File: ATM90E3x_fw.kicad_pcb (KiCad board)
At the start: 2 copper layers, 50.8 x 50.8 mm, 67 parts, among them IC1 ATM90E36_ATM90E36, J1 RJ45, J2 CONN_01X04, J3 GS3, J4 GS3, J5 GS3, J6 CONN_01X06, J7 CONN_01X06, J8 CONN_01X04, J9 GROVE-SMD-90D, U1 ROF-78E, Y1 Crystal_GND24

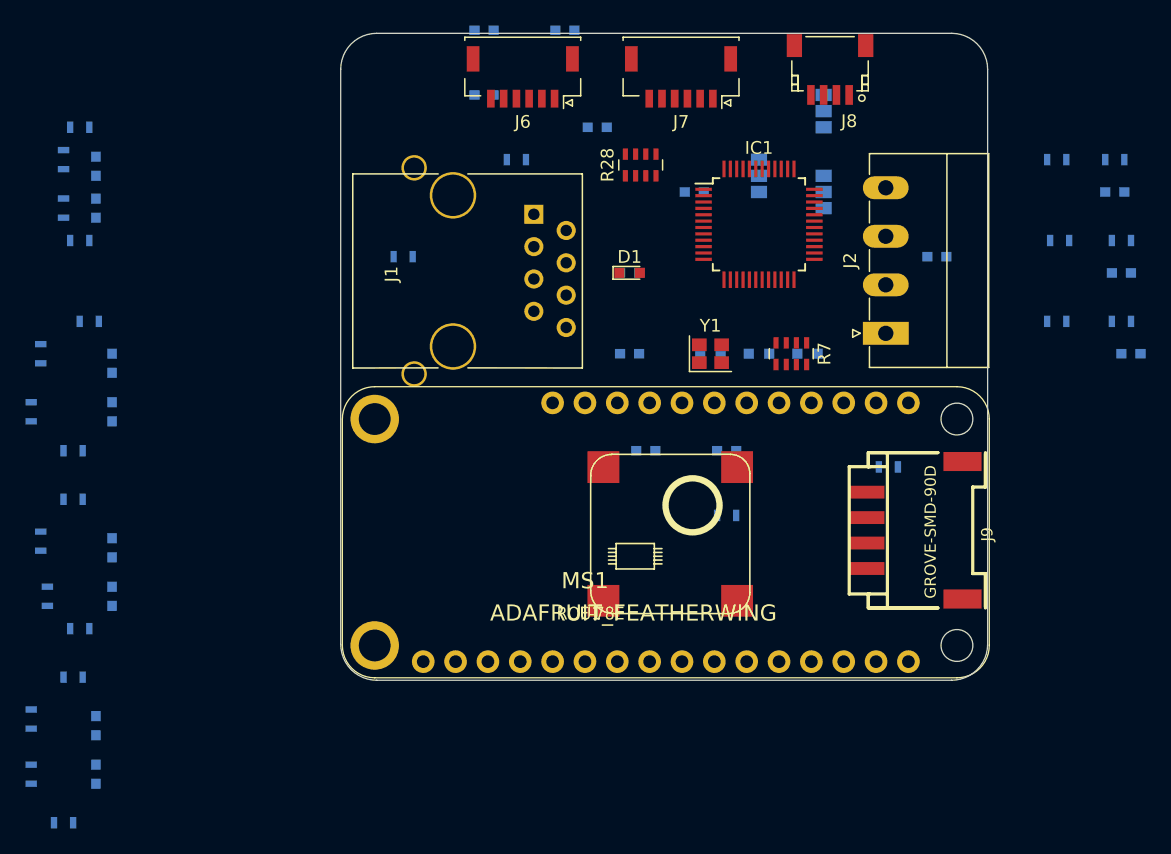
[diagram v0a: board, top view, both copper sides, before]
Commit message: Changes from freelancer on fiverr
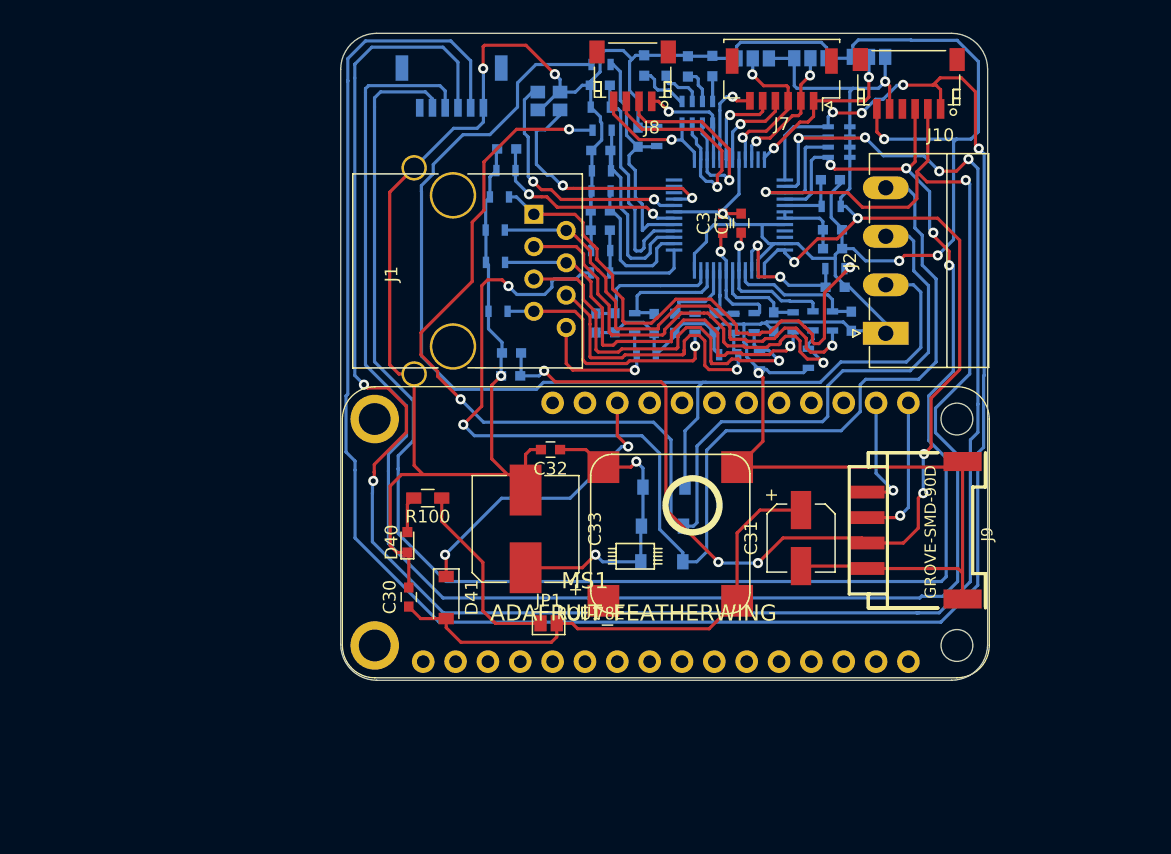
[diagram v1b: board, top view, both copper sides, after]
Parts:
- added C30: 1u/16V, Capacitors_SMD:C_0603, F.Cu at (112.2, 85.2)
- added C31: 100u/16V, Capacitors_SMD:CP_Elec_5x5.8, F.Cu at (143.0, 80.5)
- added C32: 1u/50V, Capacitors_SMD:C_0603, F.Cu at (123.3, 73.6)
- added C33: 220u/50V, Capacitors_SMD:CP_Elec_8x10, F.Cu at (121.4, 79.8)
- added D40: LED, LEDs:LED_0603, F.Cu at (112.1, 80.8)
- added D41: D_Schottky, Diodes_SMD:D_SOD-123, F.Cu at (115.1, 85.2)
- added D42: D_Schottky, Diodes_SMD:D_SOD-123, B.Cu at (132.1, 82.4)
- added D43: D_Schottky, Diodes_SMD:D_SOD-123, B.Cu at (132.1, 79.6)
- added D44: D_Schottky, Diodes_SMD:D_SOD-123, B.Cu at (132.2, 76.5)
- added J10: CONN_01X06, Connectors_JST:JST_SH_SM06B-SRSS-TB_06x1.00mm_Angled, F.Cu at (151.5, 44.9)
- added JP1: Jumper_NC_Small, Connectors:GS2, F.Cu at (123.2, 87.2)
- added R100: R, Resistors_SMD:R_0603_HandSoldering, F.Cu at (113.7, 77.4)
- C3, C7: moved to F.Cu
- D1, IC1, J6, R28, R7, Y1: moved to B.Cu
- moved R12 60.3 mm to (145.7, 59.4), turned to 0 degrees
- moved R16 60.3 mm to (143.6, 66.4)
- moved C2 60.0 mm to (146.9, 63.5), turned to 90 degrees
- moved R23 59.6 mm to (129.9, 63.6), turned to 270 degrees
- moved R13 59.4 mm to (145.5, 63.5), turned to 270 degrees
- moved C1 58.8 mm to (145.7, 60.8), turned to 0 degrees
- moved R19 58.5 mm to (130.8, 66.1), turned to 0 degrees
- moved R10 58.2 mm to (139.7, 66.5)
- moved R21 57.4 mm to (142.4, 63.5), turned to 270 degrees
- moved R20 56.8 mm to (143.9, 63.5), turned to 270 degrees
- moved R11 56.8 mm to (137.3, 66.1), turned to 180 degrees
- moved R15 56.7 mm to (137.7, 63.6), turned to 270 degrees
- moved C10 56.3 mm to (131.5, 63.7)
- moved R22 56.2 mm to (134.7, 63.6), turned to 270 degrees
- moved C9 55.4 mm to (133.1, 63.6), turned to 270 degrees
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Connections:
- MS1 pad 26: Net-(MS1-Pad26) -> USB
- U1 pad 2: Net-(U1-Pad2) -> GND
- U1 pad 3: Net-(MS1-Pad26) -> Net-(C30-Pad1)
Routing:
- net GND: track 0.00 -> 333.4 mm, vias 0 -> 8
- net CS: track 0.00 -> 168.3 mm, vias 0 -> 4
- net SCLK: track 0.00 -> 160.4 mm, vias 0 -> 6
- net MISO: track 0.00 -> 158.7 mm, vias 0 -> 2
- net MOSI: track 0.00 -> 140.2 mm, vias 0 -> 4
- net +3V3: track 0.00 -> 116.8 mm, vias 0 -> 8
- net UB: track 0.00 -> 98.1 mm, vias 0 -> 2
- net UA: track 0.00 -> 95.9 mm, vias 0 -> 2
- net UC: track 0.00 -> 90.3 mm
- net I1P_IN: track 0.00 -> 42.6 mm, vias 0 -> 1
- net Net-(C30-Pad1): track 0.00 -> 40.8 mm
- net I1N_IN: track 0.00 -> 37.0 mm, vias 0 -> 1
- net I2P_IN: track 0.00 -> 35.7 mm, vias 0 -> 1
- net I2N_IN: track 0.00 -> 32.8 mm, vias 0 -> 1
- net I3P_IN: track 0.00 -> 31.5 mm, vias 0 -> 1
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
